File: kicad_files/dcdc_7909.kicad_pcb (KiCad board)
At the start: 2 copper layers, 39.8 x 29.2 mm, 28 parts, among them J1 V_IN, J2 G_IN, J3 +10V, J4 G_OUT, J5 -10V, U1 TMR6, U2 LT3045xMSE, U3 LT3094xMSE

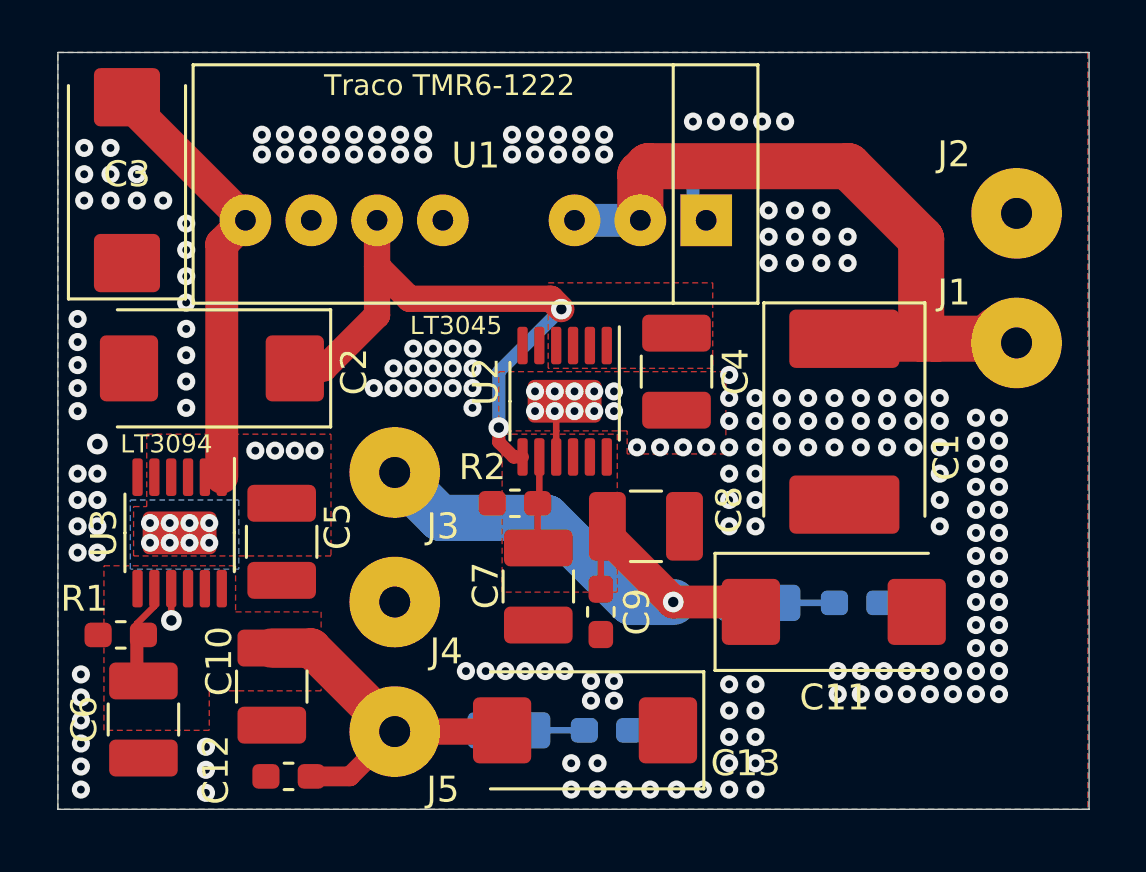
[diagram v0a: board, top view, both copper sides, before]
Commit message: v1.1
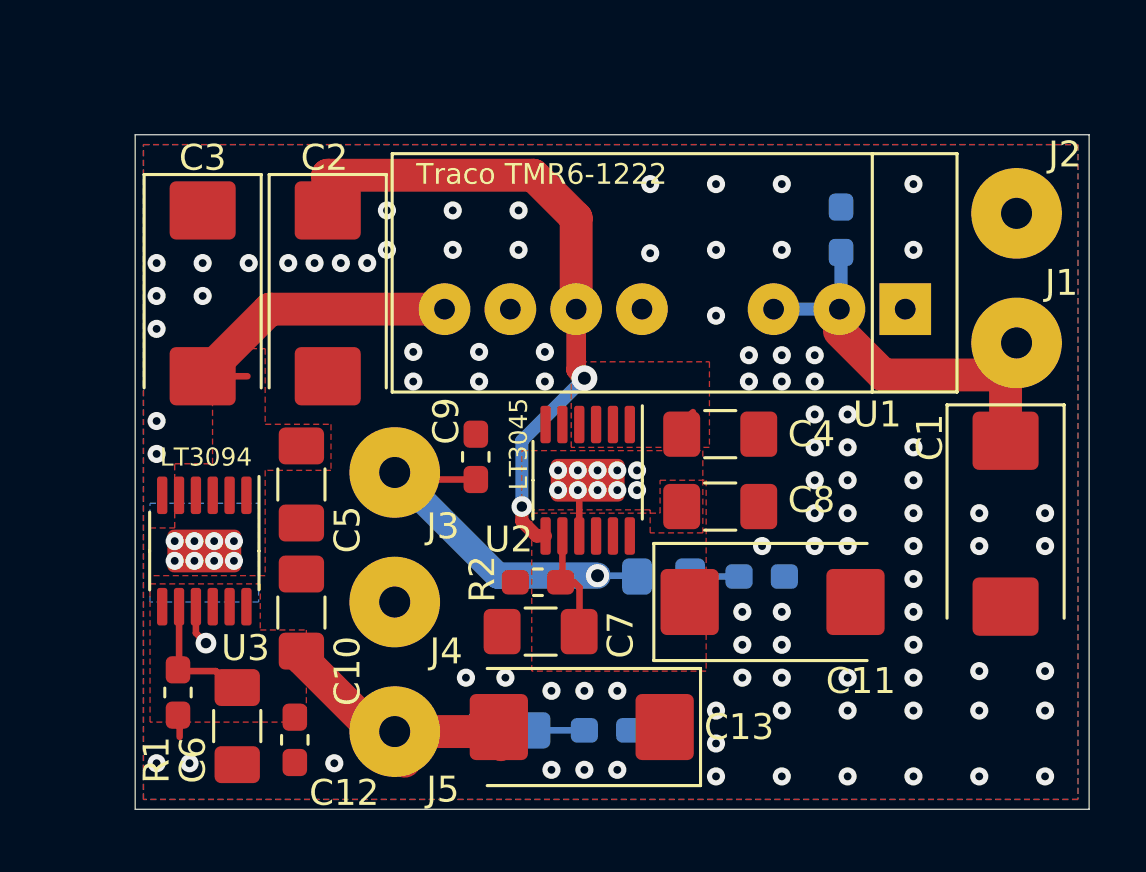
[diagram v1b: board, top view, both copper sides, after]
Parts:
- C1: footprint Capacitor_Tantalum_SMD:CP_EIA-7360-38_Kemet-E_Pad2.25x4.25mm_HandSolder -> Capacitor_Tantalum_SMD:CP_EIA-7343-31_Kemet-D_Pad2.25x2.55mm_HandSolder
- C10, C4, C5, C6, C7, C8: footprint Capacitor_SMD:C_1210_3225Metric_Pad1.42x2.65mm_HandSolder -> Capacitor_SMD:C_1206_3216Metric_Pad1.42x1.75mm_HandSolder
- C11, C2, C3: footprint Capacitor_Tantalum_SMD:CP_EIA-7343-15_Kemet-W_Pad2.25x2.55mm_HandSolder -> Capacitor_Tantalum_SMD:CP_EIA-7343-31_Kemet-D_Pad2.25x2.55mm_HandSolder
- moved U1 8.41 mm to (108.9, 60.7)
- moved C9 7.69 mm to (92.3, 66.4), turned to 90 degrees
- moved C1 7.36 mm to (112.8, 69.0)
- moved C14 7.06 mm to (106.4, 57.6), turned to 90 degrees
- moved C2 5.33 mm to (86.6, 60.1), turned to 270 degrees
- moved C3 5.25 mm to (81.8, 60.1), turned to 270 degrees
- moved R3 3.82 mm to (99.6, 71.0)
- moved D1 3.82 mm to (103.4, 71.0)
- moved C6 3.63 mm to (83.1, 76.8)
- moved U2 3.18 mm to (96.6, 67.3)
- moved R2 3.18 mm to (94.7, 71.2)
- moved R1 3.13 mm to (80.8, 75.5), turned to 270 degrees
- moved C10 3.08 mm to (85.6, 72.4), turned to 90 degrees
- moved C8 2.97 mm to (101.8, 68.3)
- moved C4 2.94 mm to (101.8, 65.5), turned to 0 degrees
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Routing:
- net VCC: track 29.3 -> 16.9 mm
- net +12V: track 24.8 -> 14.3 mm
- net Net-(C3-Pad2): track 16.9 -> 12.1 mm, vias 12 -> 8
- net -12V: track 17.6 -> 13.6 mm
- net Net-(C2-Pad1): track 23.4 -> 26.3 mm
- net GND: track 6.06 -> 4.72 mm, vias 216 -> 106
- net Net-(C6-Pad1): track 3.95 -> 5.02 mm
- net Net-(C7-Pad1): track 3.35 -> 4.01 mm
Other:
- board size 39.8 x 29.2 mm -> 36.8 x 26 mm
- board text added: "Alpine 7909 DC/DC v1.1 (c) M. Dymczyk 04.2020"
- board text removed: "Alpine 7909 DC-DC converter v1.0 +/-10V 04.2020 M. Dymczyk"
